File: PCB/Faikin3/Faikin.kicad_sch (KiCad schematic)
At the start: 33 parts, among them J1 1x5, J2 Prog, Q3 PMF250XNEX, U1 ESP32-PICO-MINI-02, U3 MD8942, U4 Barcode

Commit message: BAV99S part fix
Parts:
- D1: JLCPCB Rotation Offset (none) -> 90; LCSC Part # (none) -> C712378
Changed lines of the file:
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@@
+      (effects (font (size 1.27 1.27)) hide)
+    )
+    (property "LCSC Part #" "C712378" (at 118.11 146.05 0)
+      (effects (font (size 1.27 1.27)) hide)
+    )
+    (property "JLCPCB Rotation Offset" "90" (at 118.11 146.05 0)
       (effects (font (size 1.27 1.27)) hide)
     )
@@
       (effects (font (size 1.27 1.27)) hide)
     )
+    (property "LCSC Part #" "C712378" (at 118.11 127.635 0)
+      (effects (font (size 1.27 1.27)) hide)
+    )
+    (property "JLCPCB Rotation Offset" "90" (at 118.11 127.635 0)
+      (effects (font (size 1.27 1.27)) hide)
+    )

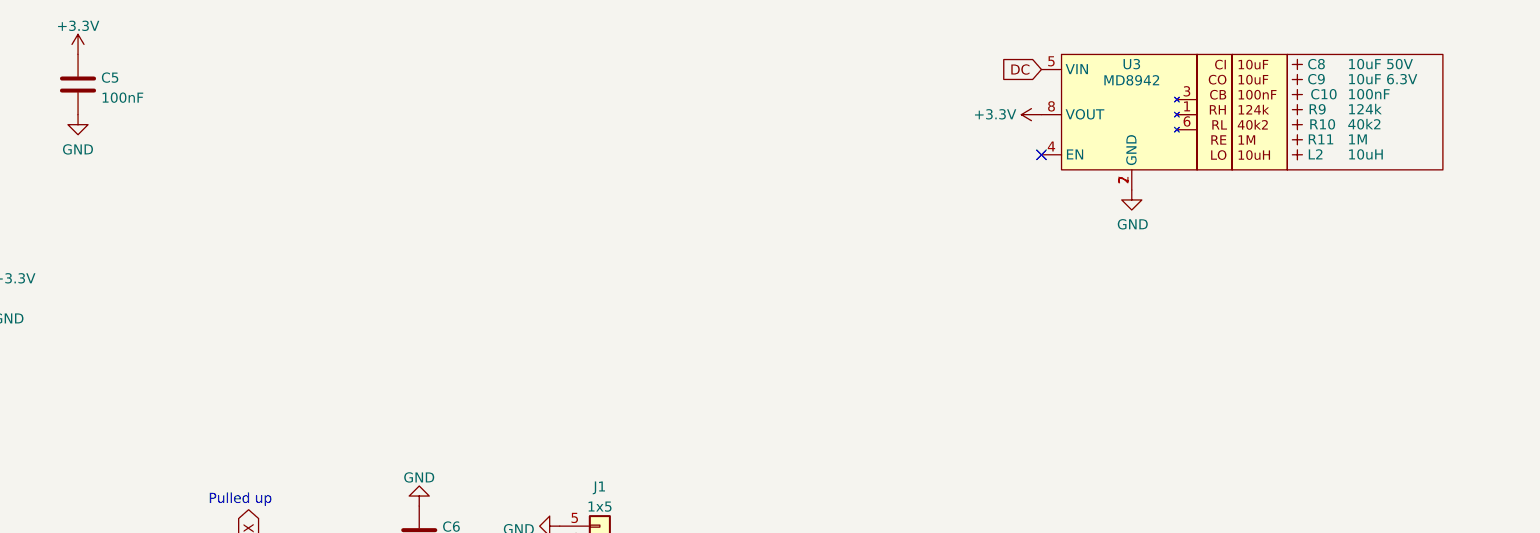
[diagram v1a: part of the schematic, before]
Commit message: V Cuts
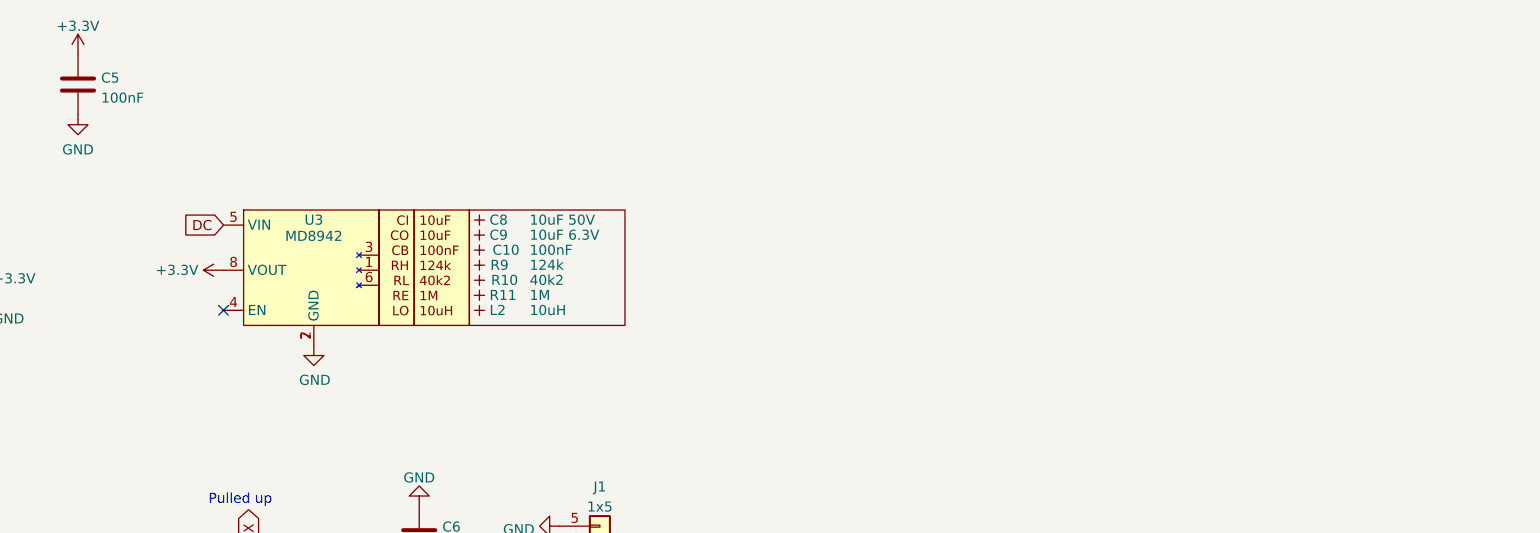
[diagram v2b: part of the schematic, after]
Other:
- moved on the sheet: C10, C8, C9, L2, R10, R11, R9, U3
